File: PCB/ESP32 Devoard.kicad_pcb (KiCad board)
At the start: 2 copper layers, 27.9 x 38.7 mm, 23 parts, among them J1 USB_C_Receptacle_USB2.0_16P, J2 Conn_01x20_Pin, J3 Conn_01x20_Pin, SW1 SW_Push, SW2 SW_Push, U2 AP63203WU, U3 ESP32-S3-WROOM-1

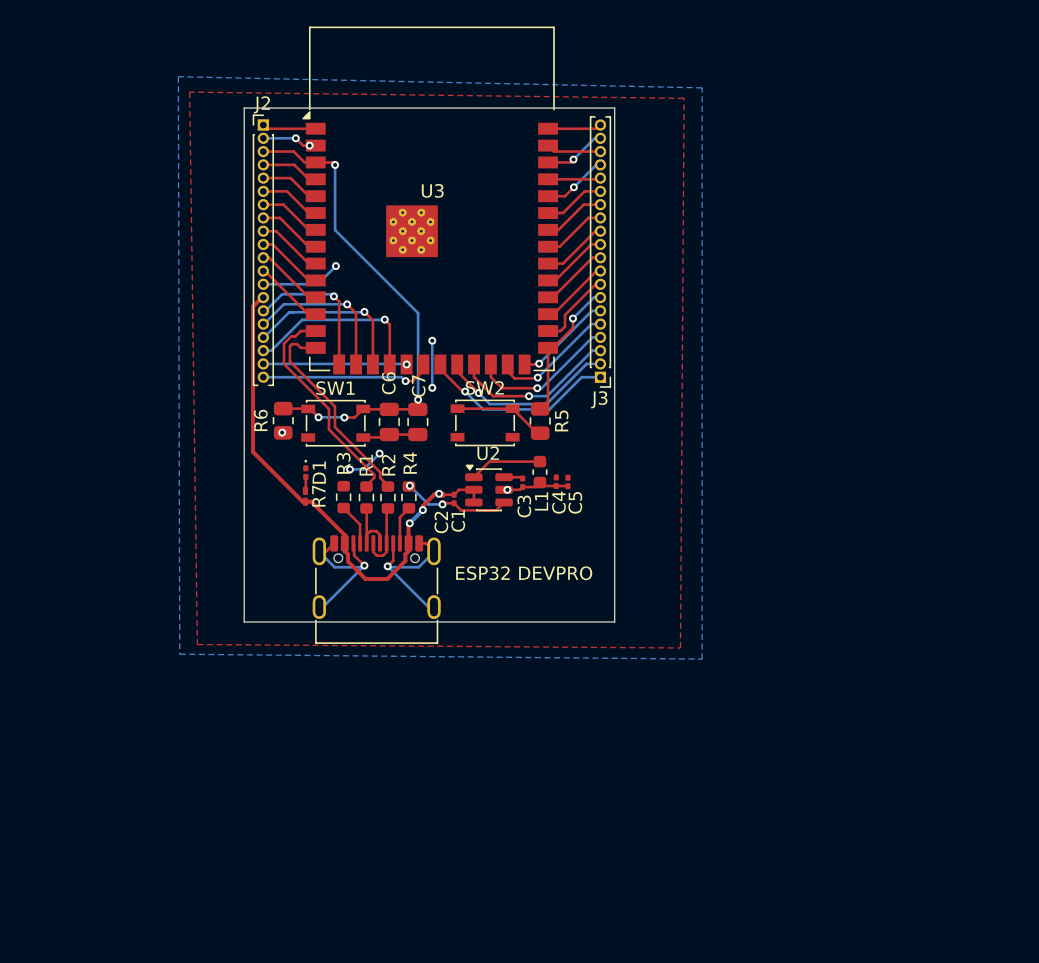
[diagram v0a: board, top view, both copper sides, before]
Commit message: Add files via upload
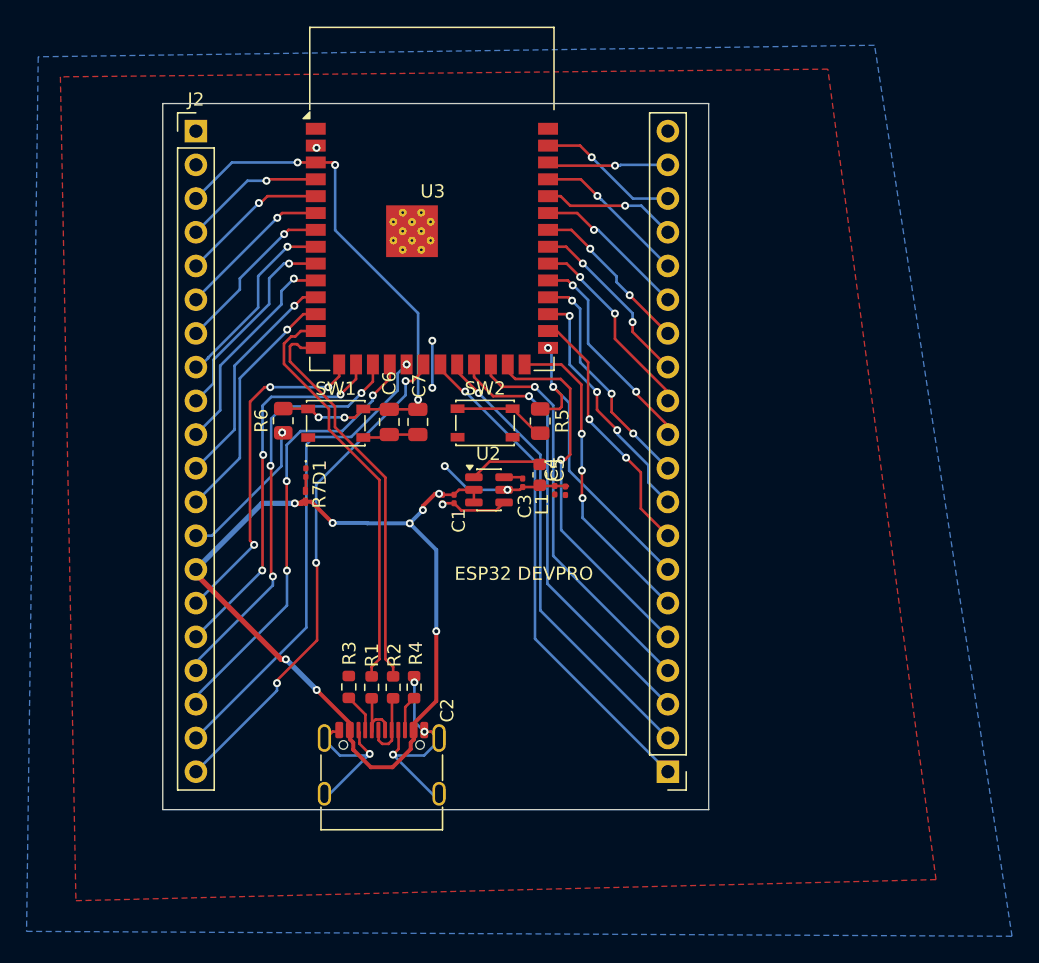
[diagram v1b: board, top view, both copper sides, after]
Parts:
- J2, J3: footprint Connector_PinHeader_1.00mm:PinHeader_1x20_P1.00mm_Vertical -> Connector_PinHeader_2.54mm:PinHeader_1x20_P2.54mm_Vertical
- moved J3 30.2 mm to (129.5, 106.7)
- moved R1 14.3 mm to (107.2, 100.3)
- moved R2 14.3 mm to (108.8, 100.3)
- moved R3 14.3 mm to (105.5, 100.3)
- moved R4 14.3 mm to (110.4, 100.3)
- moved J1 14.1 mm to (108.0, 107.3)
- moved J2 5.10 mm to (94.0, 58.4)
- moved C5 0.69 mm to (121.8, 85.5), turned to -90 degrees
- moved C4 0.65 mm to (121.0, 85.5), turned to -90 degrees
- moved L1 0.21 mm to (119.9, 84.3)
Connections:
- J1 pad SH: (no net) -> GND
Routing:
- net +5V: track 39.0 -> 68.8 mm, vias 3 -> 8
- net I011: track 10.8 -> 36.4 mm
- net I012: track 13.0 -> 38.2 mm, vias 1 -> 3
- net I013: track 14.7 -> 37.9 mm
- net I014: track 13.6 -> 34.7 mm
- net I021: track 12.5 -> 33.2 mm
- net I010: track 13.7 -> 33.5 mm, vias 1 -> 3
- net I09: track 12.6 -> 31.6 mm, vias 1 -> 3
- net I047: track 11.1 -> 30.1 mm
- net I048: track 9.42 -> 28.3 mm
- net I046: track 11.7 -> 28.5 mm, vias 1 -> 3
- net I045: track 7.39 -> 24.1 mm, vias 1 -> 3
- net _D-: track 16.6 -> 31.1 mm
- net _D+: track 15.8 -> 30.2 mm
- net I03: track 11.7 -> 25.5 mm, vias 1 -> 3
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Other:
- board size 27.9 x 38.7 mm -> 41.1 x 53.2 mm
